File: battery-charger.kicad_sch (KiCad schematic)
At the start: 12 parts, among them U4 SGM41524YTDC8G/TR

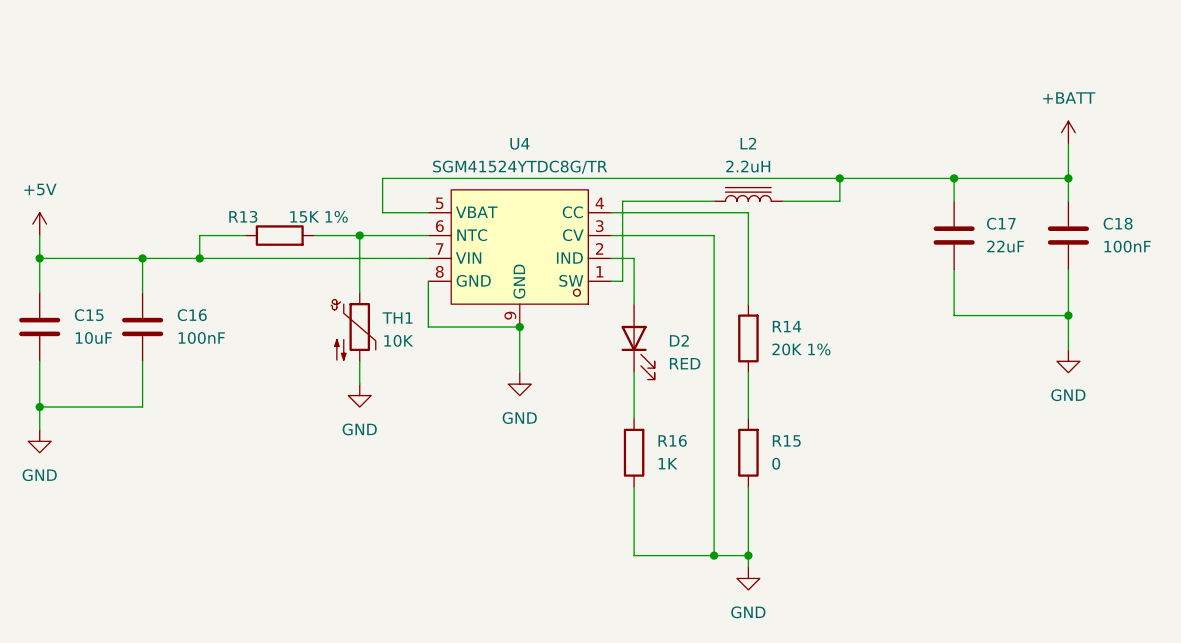
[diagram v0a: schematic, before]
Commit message: rename project
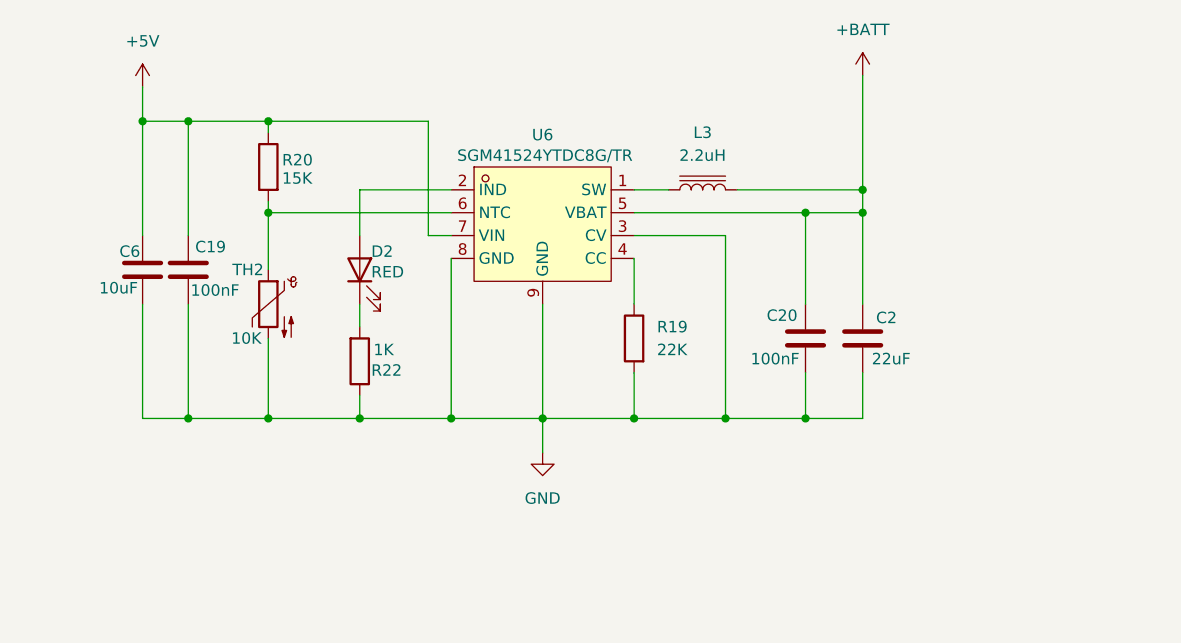
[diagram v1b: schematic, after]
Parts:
- removed C15: 10uF, symbol Device:C
- removed C16, C18: 100nF, symbol Device:C
- removed C17: 22uF, symbol Device:C
- removed L2: 2.2uH, symbol Device:L_Iron
- removed R13: 15K 1%, symbol Device:R
- removed R14: 20K 1%, symbol Device:R
- removed R15: 0, symbol Device:R
- removed R16: 1K, symbol Device:R
- removed TH1: 10K, symbol Device:Thermistor_NTC
- removed U4: SGM41524YTDC8G/TR, pager-jlc:DFN-8_L3.0-W2.0-P0.50-TL-EP-1, symbol pager-jlc:SGM41524YTDC8G_TR
- added C19, C20: 100nF, symbol Device:C
- added C2: 22uF, symbol Device:C
- added C6: 10uF, symbol Device:C
- added L3: 2.2uH, symbol Device:L_Iron
- added R19: 22K, symbol Device:R
- added R20: 15K, symbol Device:R
- added R22: 1K, symbol Device:R
- added TH2: 10K, symbol Device:Thermistor_NTC
- added U6: SGM41524YTDC8G/TR, pager-jlc:DFN-8_L3.0-W2.0-P0.50-TL-EP-1, symbol pager-jlc:SGM41524YTDC8G_TR
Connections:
- net +5V: now also C19.1, C6.2, R20.1, U6.7 (VIN)
- net +BATT: now also C2.2, C20.1, L3.1, U6.5 (VBAT)
- net GND: now also C19.2, C2.1, C20.2, C6.1, R19.2, R22.1, TH2.2, U6.3 (CV), U6.8 (GND), U6.9 (GND)
- net at D2.1 (K): now also R22.2
- net at D2.2 (A): now also U6.2 (IND)
- new net: R20.2, TH2.1, U6.6 (NTC)
- new net: L3.2, U6.1 (SW)
- new net: R19.1, U6.4 (CC)
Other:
- title: (none) -> Meshpager
